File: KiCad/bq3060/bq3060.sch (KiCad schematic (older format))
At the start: 68 parts, among them J1 Conn_01x04_Male, J2 Conn_01x03_Male, J3 Conn_01x03_Male, Q1 Si1023x, Q2 Si1023x, Q3 NDS351AN, Q4 SI4435DYTRPBF, Q5 SI4435DYTRPBF, Q6 SI4435DYTRPBF, U1 BQ29412DCT, U2 BQ3060PW

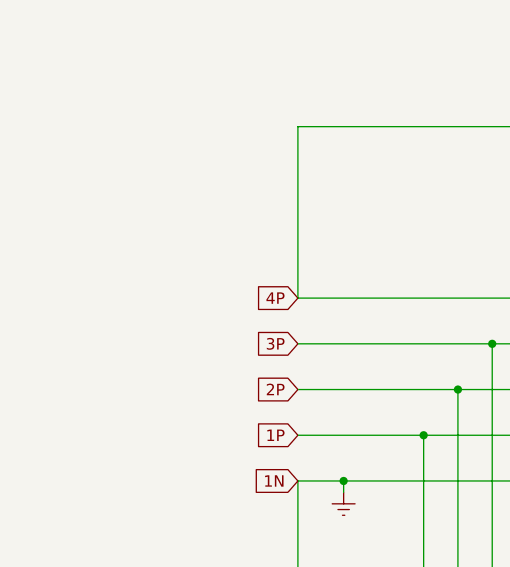
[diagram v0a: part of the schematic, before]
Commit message: Routing attempt
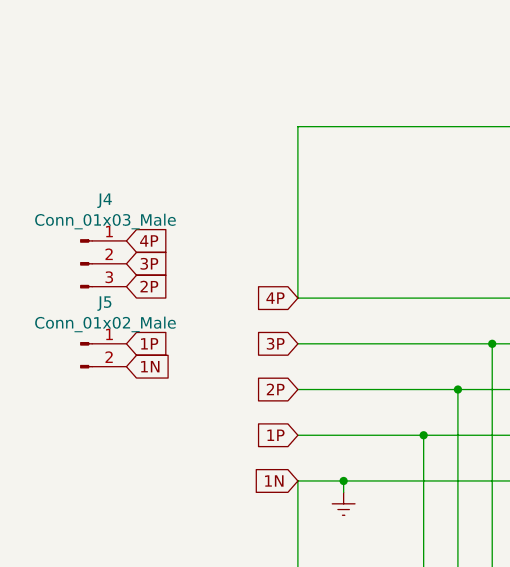
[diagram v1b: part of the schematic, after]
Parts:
- added J4: Conn_01x03_Male, Connector_Wire:SolderWirePad_1x03_P5.715mm_Drill2mm, symbol Connector:Conn_01x03_Male
- added J5: Conn_01x02_Male, Connector_Wire:SolderWirePad_1x02_P7.62mm_Drill2mm, symbol Connector:Conn_01x02_Male
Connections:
- net 1P: now also J5.1 (Pin_1)
- net 2P: now also J4.3 (Pin_3)
- net 3P: now also J4.2 (Pin_2)
- net 4P: now also J4.1 (Pin_1)
- net Earth: now also J5.2 (Pin_2)
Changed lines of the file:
@@
 Wire Wire Line
 	5050 7000 5000 7000
+Text GLabel 850  1400 2    50   Input ~ 0
+4P
+Text GLabel 850  1500 2    50   Input ~ 0
+3P
+Text GLabel 850  1600 2    50   Input ~ 0
+2P
+Text GLabel 850  1850 2    50   Input ~ 0
+1P
+Text GLabel 850  1950 2    50   Input ~ 0
+1N
+$Comp
+L Connector:Conn_01x03_Male J4
+U 1 1 60B8AEED
+P 650 1500
+F 0 "J4" H 758 1781 50  0000 C CNN
+F 1 "Conn_01x03_Male" H 758 1690 50  0000 C CNN
+F 2 "Connector_Wire:SolderWirePad_1x03_P5.715mm_Drill2mm" H 650 1500 50  0001 C CNN
+F 3 "~" H 650 1500 50  0001 C CNN
+	1    650  1500
+	1    0    0    -1
+$EndComp
+$Comp
+L Connector:Conn_01x02_Male J5
+U 1 1 60B8B6CD
+P 650 1850
+F 0 "J5" H 758 2031 50  0000 C CNN
+F 1 "Conn_01x02_Male" H 758 1940 50  0000 C CNN
+F 2 "Connector_Wire:SolderWirePad_1x02_P7.62mm_Drill2mm" H 650 1850 50  0001 C CNN
+F 3 "~" H 650 1850 50  0001 C CNN
+	1    650  1850
+	1    0    0    -1
+$EndComp
 $EndSCHEMATC
